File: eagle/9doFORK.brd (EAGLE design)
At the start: 22.6 x 35.5 mm, 39 parts, among them IC1 ATMEGA32U4-MU, SW1 SPST_TACT-KMR2, U2 SPX3819-3.3, U3 MCP73831T-2ACI/OT, X3 microUSB, Y1 32.768kHz, Y2 8MHz

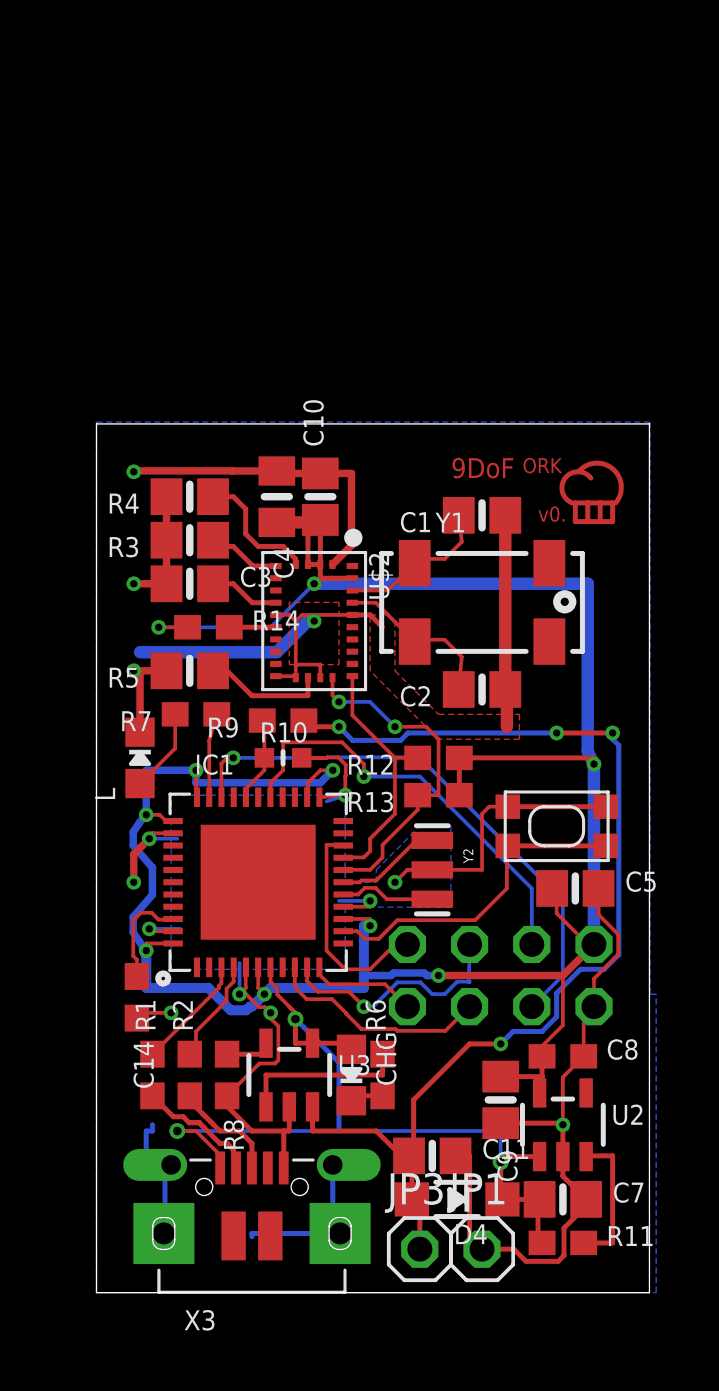
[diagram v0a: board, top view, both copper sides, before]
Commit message: fixed some bugs in rawdata-rx, working on rev 2 for board, added expenses info
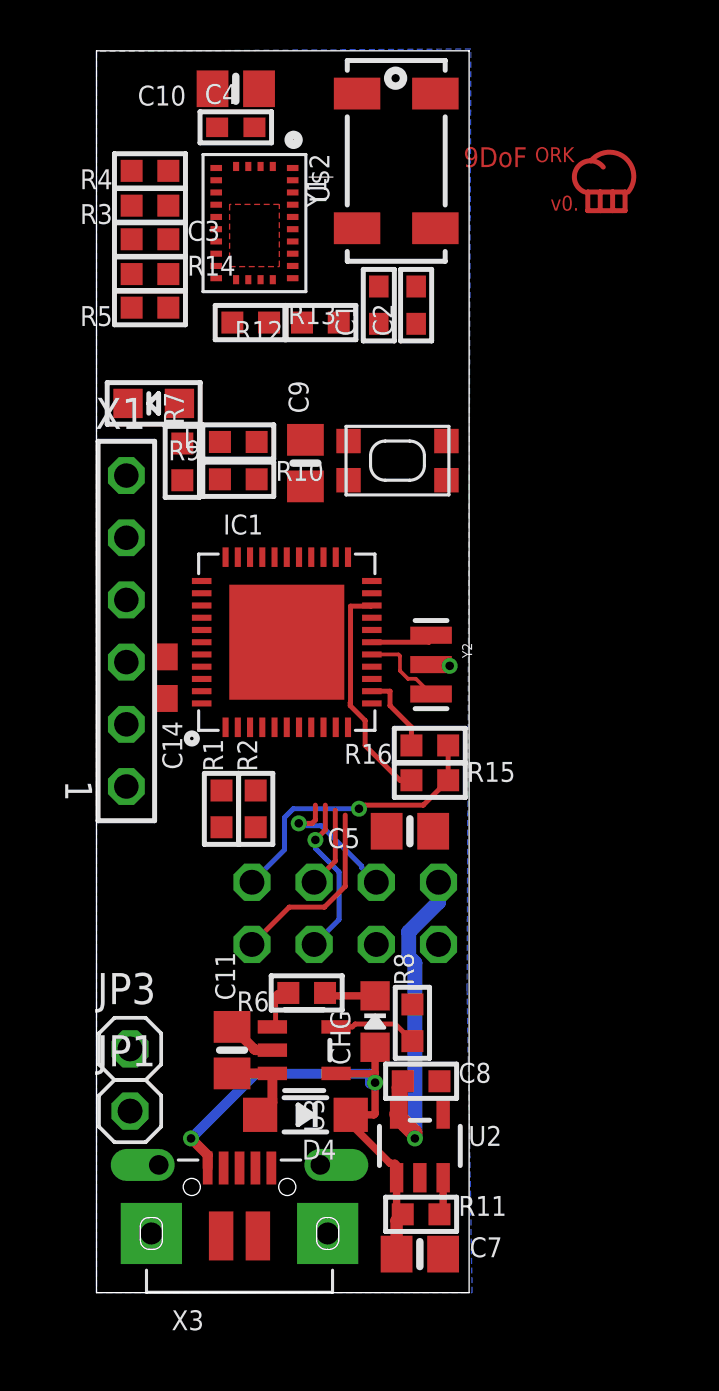
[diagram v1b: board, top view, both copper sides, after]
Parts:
- added R15, R16: 10k, microbuilder:0603-MINI
- added X1: TSW-106-02-S-S, con-samtec:TSW-106-02-S-S
- C1, C2: device microbuilder:0805-NO -> microbuilder:_0603
- C3, R3, R4, R5: device microbuilder:0805-NO -> microbuilder:0603-MINI
- C4: device microbuilder:0805_10MGAP -> microbuilder:_0603
- C8, R1, R11, R12, R13, R14, R2, R6, R7, R8, R9: device microbuilder:0603-NO -> microbuilder:0603-MINI
- L: device microbuilder:CHIPLED_0805_NOOUTLINE -> microbuilder:CHIPLED_0805
- R10: device microbuilder:_0603MP -> microbuilder:0603-MINI
- moved C9 27.2 mm to (8.53, 33.9), turned to 90 degrees
- moved R13 20.8 mm to (6.30, 39.6), turned to 0 degrees
- moved R12 18.4 mm to (9.14, 39.6)
- moved Y1 18.4 mm to (12.2, 46.2), turned to 90 degrees
- moved C10 17.0 mm to (5.69, 49.2), turned to 180 degrees
- moved U$2 16.4 mm to (6.45, 43.7)
- moved SW1 16.3 mm to (12.3, 34.0)
- moved C2 15.9 mm to (13.1, 40.3), turned to 90 degrees
- moved JP1 15.4 mm to (1.37, 7.42)
- moved C4 15.2 mm to (5.69, 47.6), turned to 0 degrees
- moved R5 14.9 mm to (2.18, 40.2)
- moved R14 14.6 mm to (2.18, 41.6)
- moved L 14.5 mm to (2.34, 36.3), turned to 90 degrees
- moved JP3 14.4 mm to (1.37, 9.96)
- moved C3 14.2 mm to (2.18, 43.0)
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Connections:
- removed net D4: IC1.25
- removed net D7: IC1.1
- new net N$13: JP2.8, R15.2, R16.1
- net A0: now also X1.6
- net A1: now also X1.5
- net A2: now also X1.4
- net A3: now also X1.3
- net A4: now also X1.2
- net A5: now also X1.1
- net CE: now also IC1.1; no longer IC1.31
- net CSN: now also IC1.8; no longer IC1.27
- net IRQ: now also R15.1; no longer JP2.8
- net RST: now also R16.2
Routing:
- net GND: track 130.5 -> 2.82 mm, vias 14 -> 1
- net +3V3: track 109.1 -> 16.4 mm, vias 10 -> 1
- net VBAT: track 45.7 -> 3.54 mm, vias 4 -> 0
- net CE: track 22.7 -> 0.00 mm, vias 1 -> 0
- net SCL_3V: track 13.9 -> 0.00 mm, vias 2 -> 0
- net VBUS: track 35.8 -> 22.8 mm, vias 3 -> 2
- net N$13: track 0.00 -> 12.0 mm, vias 0 -> 1
- net CSN: track 17.7 -> 5.73 mm
- net SDA_3V: track 10.4 -> 0.00 mm
- net RST: track 13.4 -> 3.32 mm
- net N$2: track 6.79 -> 0.00 mm
- net MOSI: track 10.0 -> 3.30 mm, vias 1 -> 0
- net N$1: track 6.38 -> 0.00 mm
- net PS1_3V: track 5.25 -> 0.00 mm
- net I2CADDR_3V: track 5.03 -> 0.00 mm
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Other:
- board size 22.6 x 35.5 mm -> 15.2 x 50.7 mm
